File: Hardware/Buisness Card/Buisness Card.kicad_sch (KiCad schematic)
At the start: 25 parts, among them J101 USB_A, J102 Conn_01x03_Male, J103 Tag Connect, U101 NCP1117-12_SOT223, U102 ATtiny85-20S, U103 ProtoBoard

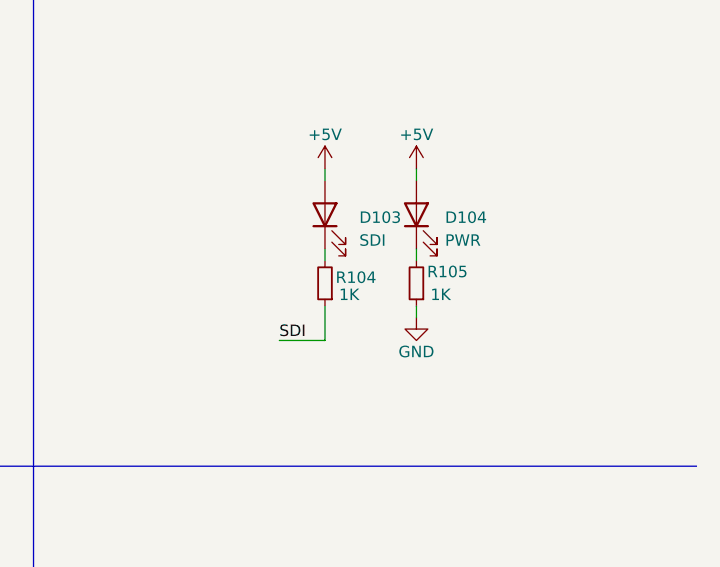
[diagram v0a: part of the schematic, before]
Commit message: Fix for #2
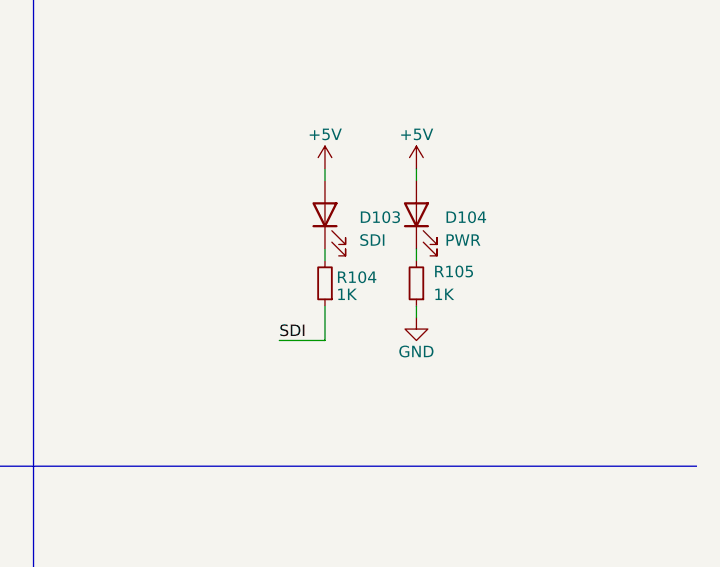
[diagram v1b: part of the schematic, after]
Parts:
- C101: LCSC# (none) -> C28323
- C102, C104: LCSC# (none) -> C138340
- C103: LCSC# (none) -> C1824
- D101, D102: LCSC# (none) -> C2891771
- D103, D104: LCSC# (none) -> C84256
- D105: LCSC# (none) -> C165467
- R101: LCSC# (none) -> C325846
- R102, R103: LCSC# (none) -> C17802
- R104, R105: LCSC# (none) -> C17513
- U102: LCSC# (none) -> C89852
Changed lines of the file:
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@@
+      (effects (font (size 1.27 1.27)) hide)
+    )
+    (property "LCSC#" "C17802" (at 66.04 93.98 90)
       (effects (font (size 1.27 1.27)) hide)
     )
@@
       (effects (font (size 1.27 1.27)) hide)
     )
+    (property "LCSC#" "C165467" (at 62.23 78.74 90)
+      (effects (font (size 1.27 1.27)) hide)
+    )
     (pin "1")
     (pin "2")
@@
     )
     (property "Datasheet" "~" (at 71.12 86.36 0)
+      (effects (font (size 1.27 1.27)) hide)
+    )
+    (property "LCSC#" "C325846" (at 71.12 86.36 0)
       (effects (font (size 1.27 1.27)) hide)
     )
@@
       (effects (font (size 1.27 1.27)) hide)
     )
+    (property "LCSC#" "C84256" (at 243.205 38.1 0)
+      (effects (font (size 1.27 1.27)) hide)
+    )
     (pin "1")
     (pin "2")
@@
   (symbol (lib_id "Device:R_Small") (at 243.205 45.72 180) (unit 1)
     (in_bom yes) (on_board yes) (dnp no)
-    (property "Reference" "R104" (at 248.92 45.085 0)
-      (effects (font (size 1.27 1.27)) (justify left))
-    )
-    (property "Value" "1K" (at 247.015 46.99 0)
-      (effects (font (size 1.27 1.27)) (justify left))
+    (property "Reference" "R104" (at 244.475 45.085 0)
+      (effects (font (size 1.27 1.27)) (justify right))
+    )
+    (property "Value" "1K" (at 244.475 46.99 0)
+      (effects (font (size 1.27 1.27)) (justify right))
     )
     (property "Footprint" "Resistor_SMD:R_0805_2012Metric" (at 243.205 45.72 0)
@@
     )
     (property "Datasheet" "~" (at 243.205 45.72 0)
+      (effects (font (size 1.27 1.27)) hide)
+    )
+    (property "LCSC#" "C17513" (at 243.205 45.72 0)
       (effects (font (size 1.27 1.27)) hide)
     )
@@
       (effects (font (size 1.27 1.27)) hide)
     )
+    (property "LCSC#" "C84256" (at 253.365 38.1 0)
+      (effects (font (size 1.27 1.27)) hide)
+    )
     (pin "1")
     (pin "2")
@@
       (effects (font (size 1.27 1.27)) hide)
     )
+    (property "LCSC#" "C2891771" (at 60.96 103.505 90)
+      (effects (font (size 1.27 1.27)) hide)
+    )
     (pin "1")
     (pin "2")
@@
     )
     (property "Datasheet" "http://ww1.microchip.com/downloads/en/DeviceDoc/atmel-2586-avr-8-bit-microcontroller-attiny25-attiny45-attiny85_datasheet.pdf" (at 136.525 102.235 0)
+      (effects (font (size 1.27 1.27)) hide)
+    )
+    (property "LCSC#" "C89852" (at 136.525 102.235 0)
       (effects (font (size 1.27 1.27)) hide)
     )
@@
       (effects (font (size 1.27 1.27)) hide)
     )
+    (property "LCSC#" "C138340" (at 153.035 76.835 0)
+      (effects (font (size 1.27 1.27)) hide)
+    )
     (pin "1")
     (pin "2")
@@
       (effects (font (size 1.27 1.27)) hide)
     )
+    (property "LCSC#" "C138340" (at 81.915 41.275 0)
+      (effects (font (size 1.27 1.27)) hide)
+    )
     (pin "1")
     (pin "2")
@@
       (effects (font (size 1.27 1.27)) hide)
     )
+    (property "LCSC#" "C28323" (at 56.515 40.64 0)
+      (effects (font (size 1.27 1.27)) hide)
+    )
     (pin "1")
     (pin "2")
@@
   (symbol (lib_id "Device:R_Small") (at 253.365 45.72 180) (unit 1)
     (in_bom yes) (on_board yes) (dnp no)
-    (property "Reference" "R105" (at 259.08 44.45 0)
-      (effects (font (size 1.27 1.27)) (justify left))
-    )
-    (property "Value" "1K" (at 257.175 46.99 0)
-      (effects (font (size 1.27 1.27)) (justify left))
+    (property "Reference" "R105" (at 255.27 44.45 0)
+      (effects (font (size 1.27 1.27)) (justify right))
+    )
+    (property "Value" "1K" (at 255.27 46.99 0)
+      (effects (font (size 1.27 1.27)) (justify right))
     )
     (property "Footprint" "Resistor_SMD:R_0805_2012Metric" (at 253.365 45.72 0)
@@
     )
     (property "Datasheet" "~" (at 253.365 45.72 0)
+      (effects (font (size 1.27 1.27)) hide)
+    )
+    (property "LCSC#" "C17513" (at 253.365 45.72 0)
       (effects (font (size 1.27 1.27)) hide)
     )
@@
       (effects (font (size 1.27 1.27)) hide)
     )
+    (property "LCSC#" "C2891771" (at 78.74 103.505 90)
+      (effects (font (size 1.27 1.27)) hide)
+    )
     (pin "1")
     (pin "2")
@@
     )
     (property "Datasheet" "~" (at 83.185 91.44 0)
+      (effects (font (size 1.27 1.27)) hide)
+    )
+    (property "LCSC#" "C17802" (at 83.185 91.44 90)
       (effects (font (size 1.27 1.27)) hide)
     )
@@
       (effects (font (size 1.27 1.27)) hide)
     )
+    (property "LCSC#" "C1824" (at 142.875 76.835 0)
+      (effects (font (size 1.27 1.27)) hide)
+    )
